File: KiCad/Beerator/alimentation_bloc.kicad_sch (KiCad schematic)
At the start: 12 parts, among them SW201 SW_DPDT_x2

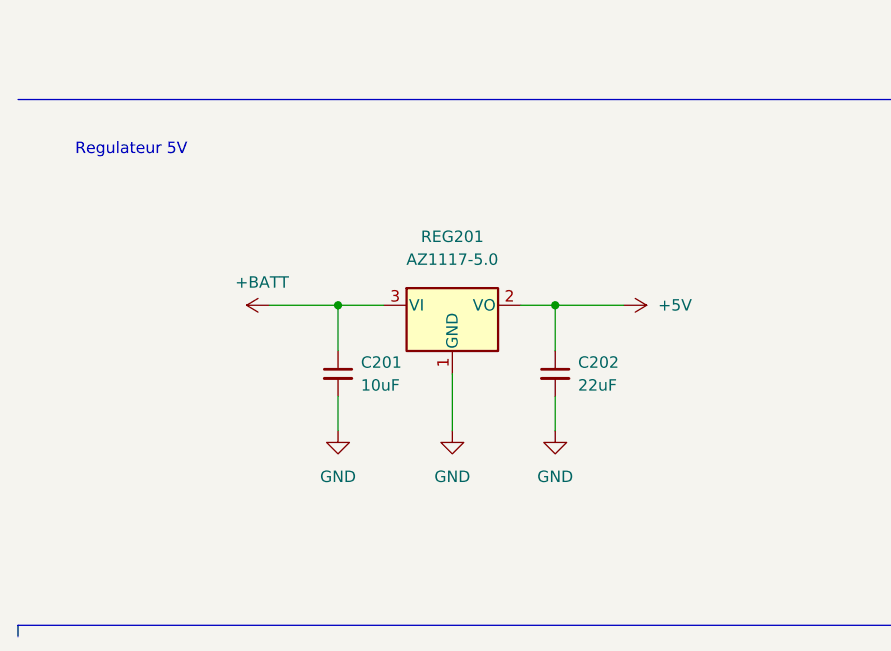
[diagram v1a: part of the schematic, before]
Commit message: version_finale_pcb
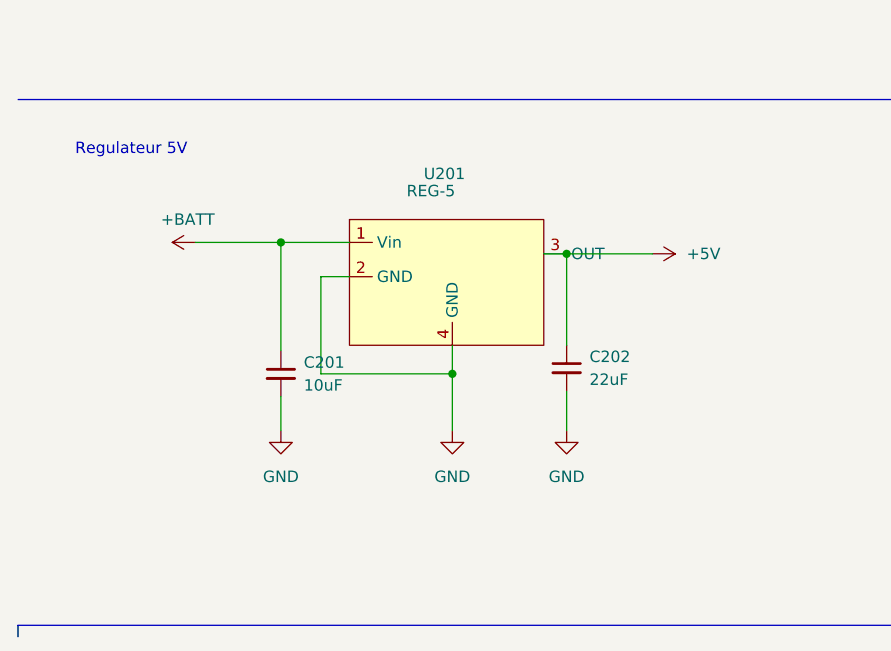
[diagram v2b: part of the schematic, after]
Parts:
- removed REG201: AZ1117-5.0, Package_TO_SOT_SMD:SOT-223, symbol Regulator_Linear:AZ1117-5.0
- added U201: REG-5, Package_TO_SOT_SMD:SOT-223, symbol Sensors_Beerator:REG-5
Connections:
- net +5V: now also U201.3 (OUT)
- net +BATT: now also U201.1 (Vin)
- net GND: now also U201.2 (GND), U201.4 (GND)
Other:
- moved on the sheet: C201, C202
